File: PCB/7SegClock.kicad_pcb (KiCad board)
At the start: 2 copper layers, 177.8 x 76.2 mm, 142 parts, among them CON1 USB-MINI-B, Q1 NPN, Q10 DMN2041LSD-13, Q11 DMN2041LSD-13, Q12 DMN2041LSD-13, Q13 DMN2041LSD-13, Q14 DMN2041LSD-13, Q15 DMN2041LSD-13, Q16 DMN2041LSD-13, Q17 DMN2041LSD-13, Q18 DMN2041LSD-13, Q19 DMN2041LSD-13, Q2 DMN2041LSD-13, Q20 DMN2041LSD-13, Q21 DMN2041LSD-13, Q22 DMN2041LSD-13, Q23 DMN2041LSD-13, Q24 DMN2041LSD-13, Q25 DMN2041LSD-13, Q26 DMN2041LSD-13, Q27 DMN2041LSD-13, Q28 DMN2041LSD-13, Q29 DMN2041LSD-13, Q3 DMN2041LSD-13, Q30 DMN2041LSD-13, Q31 DMN2041LSD-13, Q32 DMN2041LSD-13, Q4 DMN2041LSD-13, Q5 DMN2041LSD-13, Q6 DMN2041LSD-13, Q7 DMN2041LSD-13, Q8 DMN2041LSD-13, Q9 DMN2041LSD-13, U1 TPS62172DSGT, U2 P8X32A, U3 FT232RL, U4 24LC256, U5 DS3231, U6 LCMX02-640UHC-4TG144C, X1 5mhz CRYSTAL

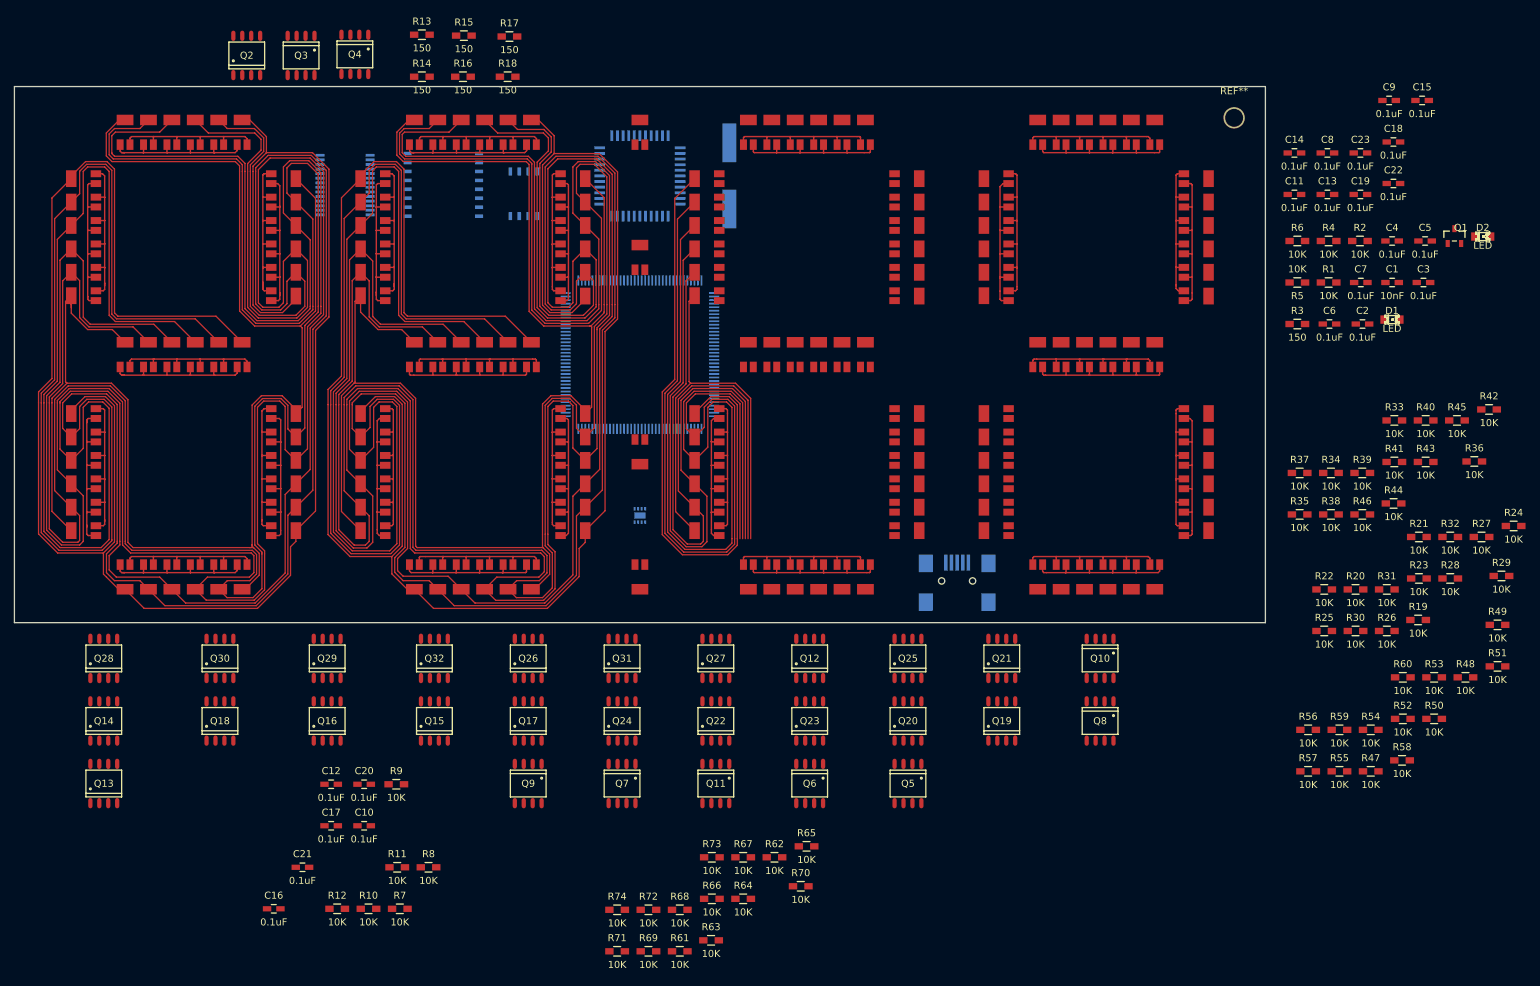
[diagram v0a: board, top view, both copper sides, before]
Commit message: PCB work.
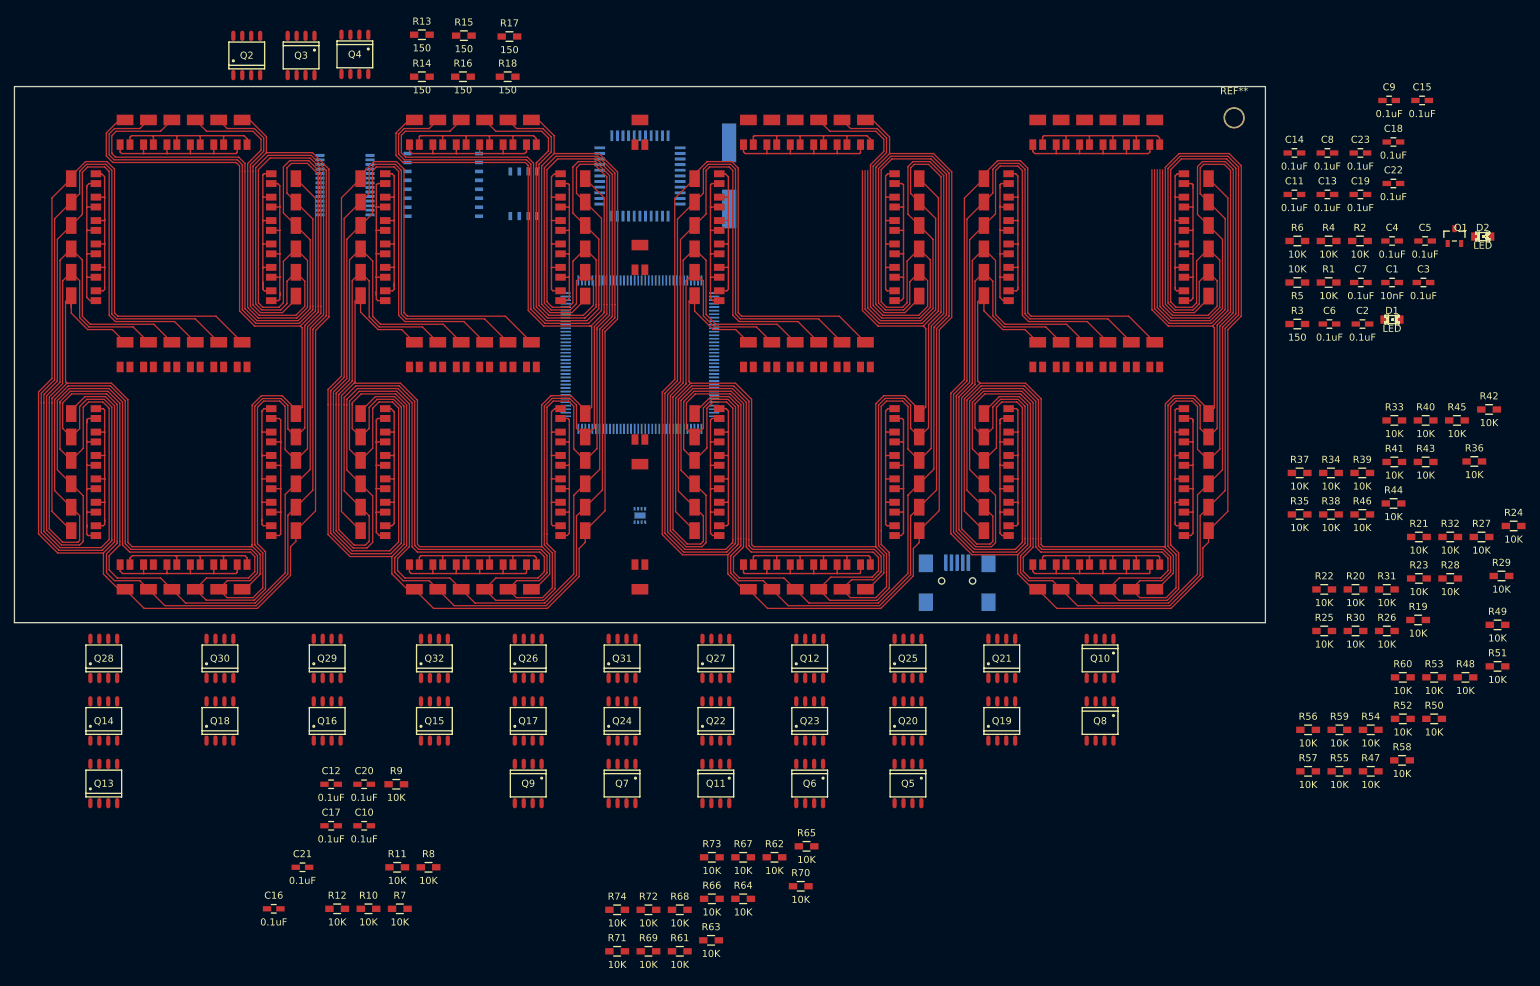
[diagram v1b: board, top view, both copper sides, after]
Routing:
- net /Lattice MACHXO2/Digit_1/A4: track 847.4 -> 1430.7 mm
- net /Lattice MACHXO2/Digit_1/A5: track 828.7 -> 1399.4 mm
- net /Lattice MACHXO2/Digit_1/A3: track 779.4 -> 1293.8 mm
- net /Lattice MACHXO2/Digit_1/A2: track 724.2 -> 1197.2 mm
- net /Lattice MACHXO2/Digit_1/A6: track 660.3 -> 1122.6 mm
- net /Lattice MACHXO2/Digit_1/A1: track 519.9 -> 848.7 mm
- net Net-(D3-Pad453): track 0.00 -> 24.6 mm
- net Net-(D3-Pad290): track 0.00 -> 24.2 mm
- net Net-(D3-Pad272): track 0.00 -> 24.2 mm
- net Net-(D3-Pad345): track 0.00 -> 24.1 mm
- net Net-(D3-Pad273): track 0.00 -> 24.1 mm
- net Net-(D3-Pad291): track 0.00 -> 24.1 mm
- net Net-(D3-Pad344): track 0.00 -> 24.0 mm
- net Net-(D3-Pad452): track 0.00 -> 23.9 mm
- net Net-(D3-Pad110): track 23.7 -> 0.00 mm
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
